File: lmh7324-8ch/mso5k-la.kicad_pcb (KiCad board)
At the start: 4 copper layers, 40 x 42 mm, 126 parts, among them IC201 lmh7324, IC401 lmh7324, J101 out, J102 in, J103 3mm, J104 3mm, J105 3mm, J106 3mm, U401 ATtiny85-20SU

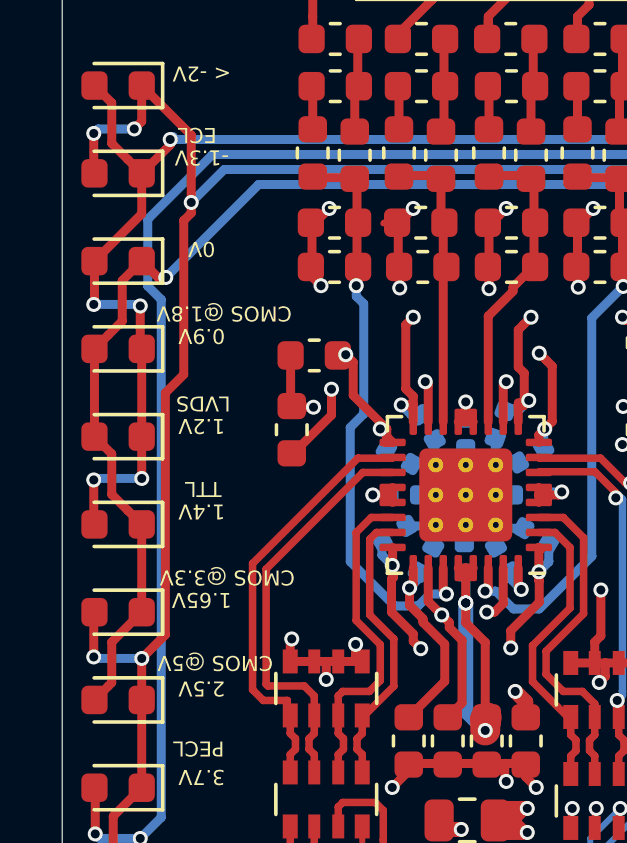
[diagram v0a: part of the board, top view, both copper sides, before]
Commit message: Added fixes for E1 and E2
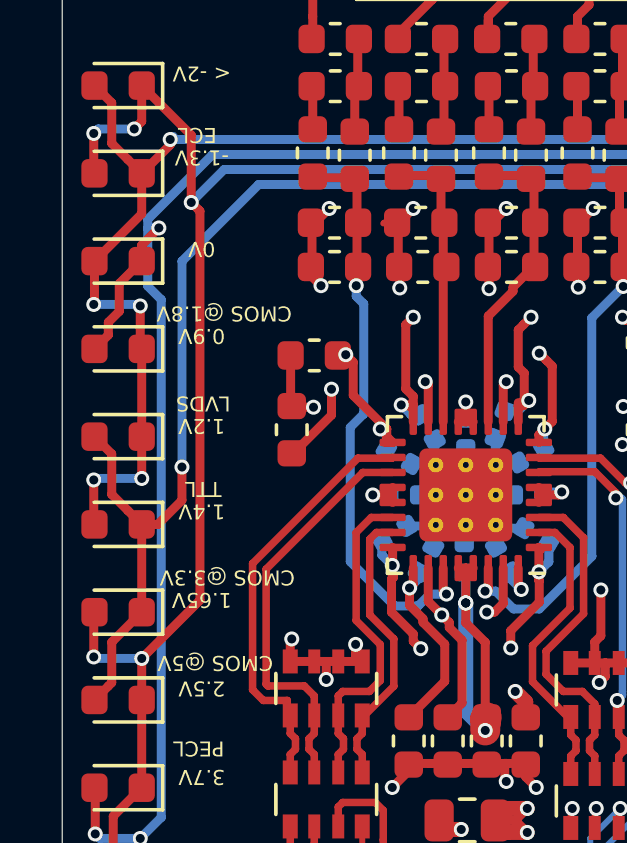
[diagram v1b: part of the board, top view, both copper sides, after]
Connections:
- D407 pad 2: Net-(D403-Pad2) -> Net-(D401-Pad1)
- D408 pad 1: Net-(D403-Pad2) -> Net-(D401-Pad1)
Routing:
- net Net-(D401-Pad1): track 60.2 -> 65.5 mm, vias 3 -> 4
- net Net-(D403-Pad2): track 51.8 -> 53.2 mm
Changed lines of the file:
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@@
     (thickness 1.6)
     (drawings 34)
-    (tracks 1692)
+    (tracks 1699)
     (zones 0)
     (modules 126)
@@
     (fp_line (start 0.8 -0.4) (end -0.5 -0.4) (layer F.Fab) (width 0.1))
     (pad 2 smd roundrect (at 0.7875 0 180) (size 0.875 0.95) (layers F.Cu F.Paste F.Mask) (roundrect_rratio 0.25)
-      (net 72 "Net-(D403-Pad2)"))
+      (net 71 "Net-(D401-Pad1)"))
     (pad 1 smd roundrect (at -0.7875 0 180) (size 0.875 0.95) (layers F.Cu F.Paste F.Mask) (roundrect_rratio 0.25)
       (net 73 "Net-(D405-Pad2)"))
@@
     )
     (pad 1 smd roundrect (at -0.7875 0 180) (size 0.875 0.95) (layers F.Cu F.Paste F.Mask) (roundrect_rratio 0.25)
-      (net 72 "Net-(D403-Pad2)"))
+      (net 71 "Net-(D401-Pad1)"))
     (pad 2 smd roundrect (at 0.7875 0 180) (size 0.875 0.95) (layers F.Cu F.Paste F.Mask) (roundrect_rratio 0.25)
       (net 73 "Net-(D405-Pad2)"))
@@
   (segment (start 33.125 32.025) (end 36.175 32.025) (width 1) (layer 3_Misc) (net 1))
   (segment (start 36.175 32.025) (end 37.575 32.025) (width 1) (layer 3_Misc) (net 1))
-  (via (at 41.8 48.3) (size 0.5) (drill 0.3) (layers F.Cu B.Cu) (net 1) (status 1000000))
+  (via (at 41.8 48.3) (size 0.5) (drill 0.3) (layers F.Cu B.Cu) (net 1))
   (via (at 42.655 53.5) (size 1) (drill 0.6) (layers F.Cu B.Cu) (net 1))
   (segment (start 41.8 48.3) (end 42.1 48.3) (width 0.3) (layer F.Cu) (net 1) (status 20))
@@
   (segment (start 18.55 41.881928) (end 18.574213 41.857715) (width 0.3) (layer F.Cu) (net 70) (status 30))
   (segment (start 18.55 43.35) (end 18.55 41.881928) (width 0.3) (layer F.Cu) (net 70) (status 20))
-  (segment (start 20.15 43.4) (end 20.936723 42.613277) (width 0.3) (layer F.Cu) (net 70))
   (segment (start 18.7 25.75) (end 18.55 25.9) (width 0.3) (layer B.Cu) (net 70))
   (segment (start 19.9 25.75) (end 18.7 25.75) (width 0.3) (layer B.Cu) (net 70))
   (via (at 21.8 28.2) (size 0.5) (drill 0.3) (layers F.Cu B.Cu) (net 70))
-  (segment (start 21.8 28.553553) (end 21.55 28.803553) (width 0.3) (layer F.Cu) (net 70))
-  (segment (start 21.8 28.2) (end 21.8 28.553553) (width 0.3) (layer F.Cu) (net 70))
-  (segment (start 21.55 33.936723) (end 20.936723 34.55) (width 0.3) (layer F.Cu) (net 70))
-  (segment (start 21.55 28.803553) (end 21.55 33.936723) (width 0.3) (layer F.Cu) (net 70))
-  (segment (start 20.936723 42.613277) (end 20.936723 34.55) (width 0.3) (layer F.Cu) (net 70))
   (segment (start 21.8 25.954968) (end 20.149213 24.304181) (width 0.3) (layer F.Cu) (net 70) (status 20))
   (segment (start 21.8 28.2) (end 21.8 25.954968) (width 0.3) (layer F.Cu) (net 70))
@@
   (segment (start 21.8 28.2) (end 22.898227 27.101773) (width 0.3) (layer B.Cu) (net 70))
   (segment (start 22.898227 27.101773) (end 51.894674 27.101773) (width 0.3) (layer B.Cu) (net 70))
+  (segment (start 22.090002 41.459998) (end 22.090002 28.490002) (width 0.3) (layer F.Cu) (net 70))
+  (segment (start 20.15 43.4) (end 22.090002 41.459998) (width 0.3) (layer F.Cu) (net 70))
+  (segment (start 22.049999 28.449999) (end 21.8 28.2) (width 0.3) (layer F.Cu) (net 70))
+  (segment (start 22.090002 28.490002) (end 22.049999 28.449999) (width 0.3) (layer F.Cu) (net 70))
   (segment (start 53.5125 25) (end 52.975 25) (width 0.3) (layer F.Cu) (net 71) (status 10))
   (via (at 52.45 25) (size 0.5) (drill 0.3) (layers F.Cu B.Cu) (net 71))
@@
   (segment (start 22.510234 26.601762) (end 50.848238 26.601762) (width 0.3) (layer B.Cu) (net 71))
   (segment (start 20.799989 48.700011) (end 20.799989 31.438001) (width 0.3) (layer B.Cu) (net 71))
-  (segment (start 20.349989 30.988001) (end 20.349989 28.762007) (width 0.3) (layer B.Cu) (net 71))
   (segment (start 20.799989 31.438001) (end 20.349989 30.988001) (width 0.3) (layer B.Cu) (net 71))
   (segment (start 20.1 49.4) (end 20.799989 48.700011) (width 0.3) (layer B.Cu) (net 71))
+  (segment (start 19.035825 32.619336) (end 19.035825 32.194175) (width 0.3) (layer F.Cu) (net 71))
+  (segment (start 18.574213 33.080948) (end 19.035825 32.619336) (width 0.3) (layer F.Cu) (net 71))
+  (segment (start 19.035825 32.194175) (end 19.4 31.83) (width 0.3) (layer F.Cu) (net 71))
+  (segment (start 19.4 30.904572) (end 20.149213 30.155359) (width 0.3) (layer F.Cu) (net 71))
+  (segment (start 19.4 31.83) (end 19.4 30.904572) (width 0.3) (layer F.Cu) (net 71))
+  (via (at 20.72 29.05) (size 0.5) (drill 0.3) (layers F.Cu B.Cu) (net 71))
+  (segment (start 20.149213 30.155359) (end 20.149213 29.620787) (width 0.3) (layer F.Cu) (net 71))
+  (segment (start 20.149213 29.620787) (end 20.72 29.05) (width 0.3) (layer F.Cu) (net 71))
+  (segment (start 20.366447 29.05) (end 20.349989 29.066458) (width 0.3) (layer B.Cu) (net 71))
+  (segment (start 20.72 29.05) (end 20.366447 29.05) (width 0.3) (layer B.Cu) (net 71))
+  (segment (start 20.349989 30.988001) (end 20.349989 29.07) (width 0.3) (layer B.Cu) (net 71))
+  (segment (start 20.349989 29.066458) (end 20.349989 29.07) (width 0.3) (layer B.Cu) (net 71))
+  (segment (start 20.349989 29.07) (end 20.349989 28.762007) (width 0.3) (layer B.Cu) (net 71))
   (segment (start 53.4125 28.75) (end 52.875 28.75) (width 0.3) (layer F.Cu) (net 72) (status 10))
   (via (at 52.45 28.75) (size 0.5) (drill 0.3) (layers F.Cu B.Cu) (net 72))
   (segment (start 52.875 28.75) (end 52.45 28.75) (width 0.3) (layer F.Cu) (net 72))
-  (segment (start 18.574213 33.080948) (end 18.574213 36.006537) (width 0.3) (layer F.Cu) (net 72) (status 30))
   (segment (start 20.149213 38.932126) (end 20.149213 41.857715) (width 0.3) (layer F.Cu) (net 72) (status 30))
-  (segment (start 19.499999 32.155162) (end 19.035825 32.619336) (width 0.3) (layer F.Cu) (net 72))
-  (segment (start 19.035825 32.619336) (end 18.574213 33.080948) (width 0.3) (layer F.Cu) (net 72) (status 20))
-  (segment (start 19.499999 30.804573) (end 19.499999 32.155162) (width 0.3) (layer F.Cu) (net 72))
-  (segment (start 20.149213 30.155359) (end 19.499999 30.804573) (width 0.3) (layer F.Cu) (net 72) (status 10))
   (segment (start 19.687601 38.470514) (end 20.149213 38.932126) (width 0.3) (layer F.Cu) (net 72) (status 20))
   (segment (start 18.574213 36.006537) (end 19.150001 36.582325) (width 0.3) (layer F.Cu) (net 72) (status 10))
@@
   (segment (start 20.149213 41.857715) (end 19.150001 42.856927) (width 0.3) (layer F.Cu) (net 72) (status 10))
   (segment (start 19.035825 44.321692) (end 18.574213 44.783304) (width 0.3) (layer F.Cu) (net 72) (status 20))
-  (segment (start 20.149213 30.155359) (end 20.693854 30.7) (width 0.3) (layer F.Cu) (net 72) (status 10))
-  (segment (start 20.693854 30.7) (end 20.94999 30.7) (width 0.3) (layer F.Cu) (net 72))
-  (via (at 20.94999 30.7) (size 0.5) (drill 0.3) (layers F.Cu B.Cu) (net 72))
   (segment (start 51.301782 27.601782) (end 52.200001 28.500001) (width 0.3) (layer B.Cu) (net 72))
   (segment (start 52.200001 28.500001) (end 52.45 28.75) (width 0.3) (layer B.Cu) (net 72))
-  (segment (start 20.94999 30.7) (end 24.048208 27.601782) (width 0.3) (layer B.Cu) (net 72))
   (segment (start 24.048208 27.601782) (end 51.301782 27.601782) (width 0.3) (layer B.Cu) (net 72))
+  (segment (start 20.686713 38.932126) (end 21.49 38.128839) (width 0.3) (layer F.Cu) (net 72))
+  (segment (start 20.149213 38.932126) (end 20.686713 38.932126) (width 0.3) (layer F.Cu) (net 72))
+  (segment (start 21.49 38.128839) (end 21.49 37.02) (width 0.3) (layer F.Cu) (net 72))
+  (via (at 21.49 37.02) (size 0.5) (drill 0.3) (layers F.Cu B.Cu) (net 72))
+  (segment (start 21.49 30.15999) (end 24.048208 27.601782) (width 0.3) (layer B.Cu) (net 72))
+  (segment (start 21.49 37.02) (end 21.49 30.15999) (width 0.3) (layer B.Cu) (net 72))
   (segment (start 53.5125 23.1) (end 52.975 23.1) (width 0.3) (layer F.Cu) (net 73) (status 10))
   (via (at 52.45 23.1) (size 0.5) (drill 0.3) (layers F.Cu B.Cu) (net 73))

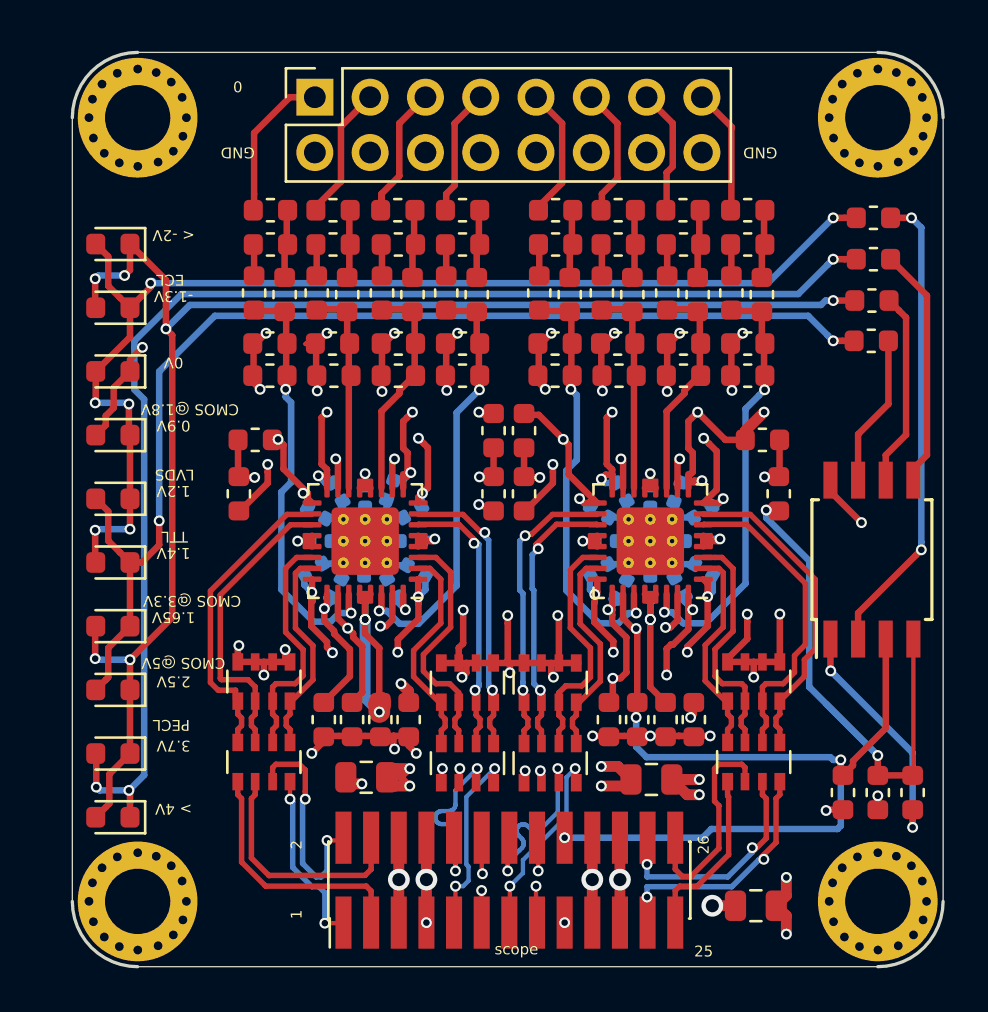
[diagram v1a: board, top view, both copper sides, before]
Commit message: Cleaning up
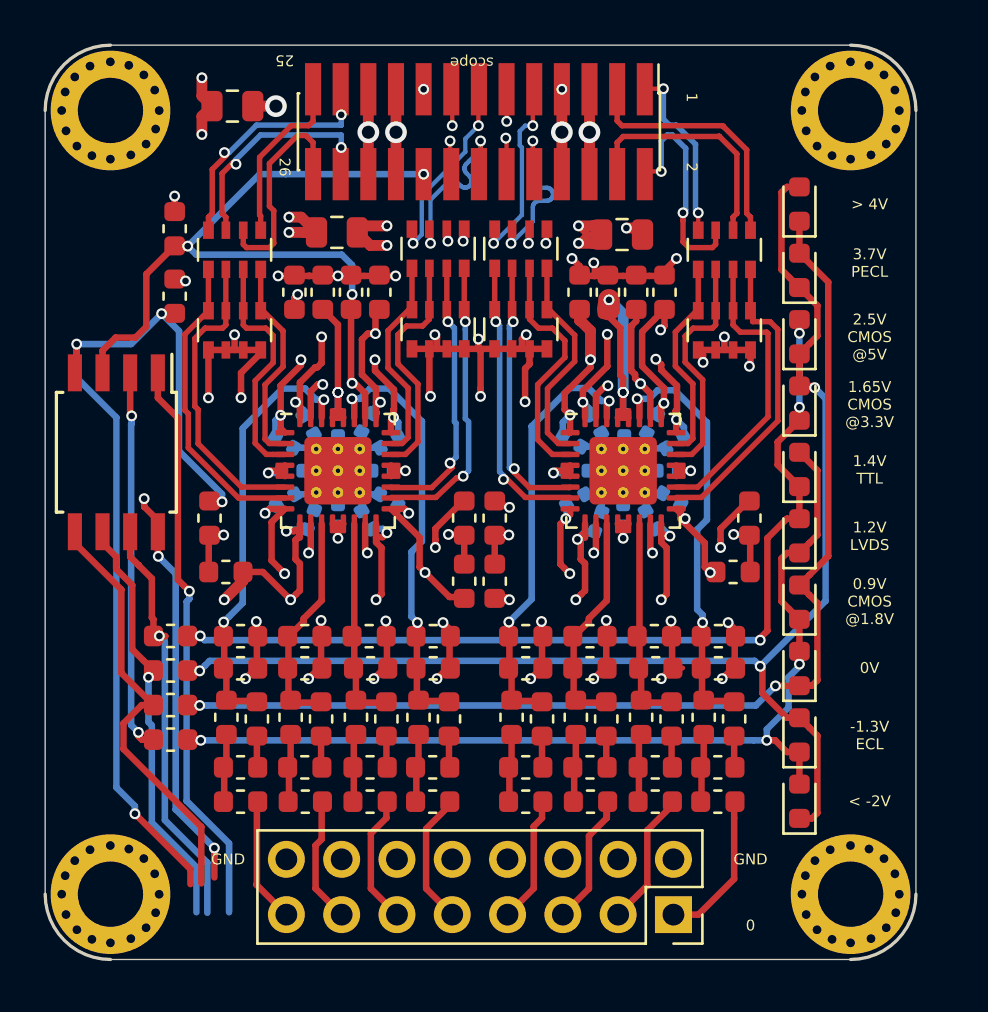
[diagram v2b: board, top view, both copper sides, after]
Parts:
- removed G***: LOGO, lmh7324-8ch:qrcode
- removed R417: 10k, Resistor_SMD:R_0603_1608Metric
- moved J106 50.6 mm to (19.3, 18.2), turned to 180 degrees
- moved J103 50.1 mm to (19.3, 54.2), turned to 180 degrees
- moved J104 48.9 mm to (53.3, 18.2), turned to 180 degrees
- moved J105 48.4 mm to (53.3, 54.2), turned to 180 degrees
- moved C102 43.9 mm to (24.9, 18.0), turned to 180 degrees
- moved D401 42.3 mm to (50.9, 22.5), turned to 90 degrees
- moved J102 41.0 mm to (45.1, 55.1), turned to 270 degrees
- moved D410 40.6 mm to (50.9, 49.9), turned to 90 degrees
- moved R421 40.2 mm to (22.0, 47.1), turned to 180 degrees
- moved C104 40.2 mm to (22.2, 23.6), turned to 90 degrees
- moved C417 39.5 mm to (22.2, 26.7), turned to 270 degrees
- moved D402 38.6 mm to (50.9, 25.5), turned to 90 degrees
- moved R418 38.2 mm to (22.0, 45.5), turned to 180 degrees
- moved D409 37.1 mm to (50.9, 46.9), turned to 90 degrees
- moved R419 36.4 mm to (22.0, 43.9), turned to 180 degrees
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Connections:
- net Net-(D401-Pad1) renamed /LEDs/PB0
- net Net-(D401-Pad2) renamed /LEDs/PB1
- net Net-(D403-Pad2) renamed /LEDs/PB2
- net Net-(D405-Pad2) renamed /LEDs/PB3
- U401 pad 1: Net-(R417-Pad1) -> ~Reset
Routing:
- net +4V: track 86.4 -> 127.4 mm, vias 19 -> 21
- net ~Reset: track 0.00 -> 26.2 mm, vias 0 -> 1
- net -2V5: track 118.2 -> 135.9 mm, vias 16 -> 18
- net /LEDs/PB0: track 65.5 -> 52.0 mm, vias 4 -> 2
- net Net-(R420-Pad2): track 6.98 -> 19.4 mm, vias 0 -> 1
- net +2V5: track 155.6 -> 166.9 mm, vias 22 -> 23
- net Net-(R417-Pad1): track 11.0 -> 0.00 mm, vias 2 -> 0
- net Net-(R419-Pad2): track 8.96 -> 19.5 mm, vias 0 -> 1
- net /LEDs/PB2: track 53.2 -> 43.0 mm, vias 2 -> 4
- net /LEDs/PB3: track 54.4 -> 45.4 mm, vias 6 -> 3
- net Net-(R418-Pad2): track 11.1 -> 20.0 mm
- net /LEDs/PB1: track 68.2 -> 61.5 mm, vias 6 -> 3
- net Vref: track 128.5 -> 122.9 mm
- net Net-(R421-Pad2): track 21.7 -> 17.6 mm
- net /Ch 4-7/C+: track 14.6 -> 13.9 mm
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- removed copper zone on 3_Misc, net +4V
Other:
- board text added: "+"
- board text added: "-"
- board text added: "-1.3V ECL"
- board text added: "0.9V CMOS @1.8V"
- board text added: "1.2V LVDS"
- board text added: "1.4V TTL"
- board text added: "1.65V CMOS @3.3V"
- board text added: "2.5V CMOS @5V"
- board text added: "3.7V PECL"
- board text added: "MISO"
- board text added: "MOSI"
- board text added: "SCK"
- board text added: "~RESET"
- board text removed: "-1.3V"
- board text removed: "0.9V"
- board text removed: "1.2V"
- board text removed: "1.4V"
- board text removed: "1.65V"
- board text removed: "2.5V"
- board text removed: "3.7V"
- board text removed: "CMOS @1.8V"
- board text removed: "CMOS @3.3V"
- board text removed: "CMOS @5V"
- board text removed: "ECL"
- board text removed: "LVDS"
- board text removed: "PECL"
- board text removed: "TTL"
